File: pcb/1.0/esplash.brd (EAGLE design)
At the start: 101 x 71.1 mm, 64 parts, among them IC1 ACS712, K1 SRD-05VDC-SL-C, K2 SRD-05VDC-SL-C, K3 SRD-05VDC-SL-C, K4 SRD-05VDC-SL-C, Q1 BCX70SMD, Q2 BCX70SMD, Q3 BCX70SMD, Q4 BCX70SMD, U1 ESP-WROOM-32, U2 EL817(S)(D)(TU)-V, U3 EL817(S)(D)(TU)-V, U4 EL817(S)(D)(TU)-V, U5 EL817(S)(D)(TU)-V, Y1 ECS-.327-12.5-13X

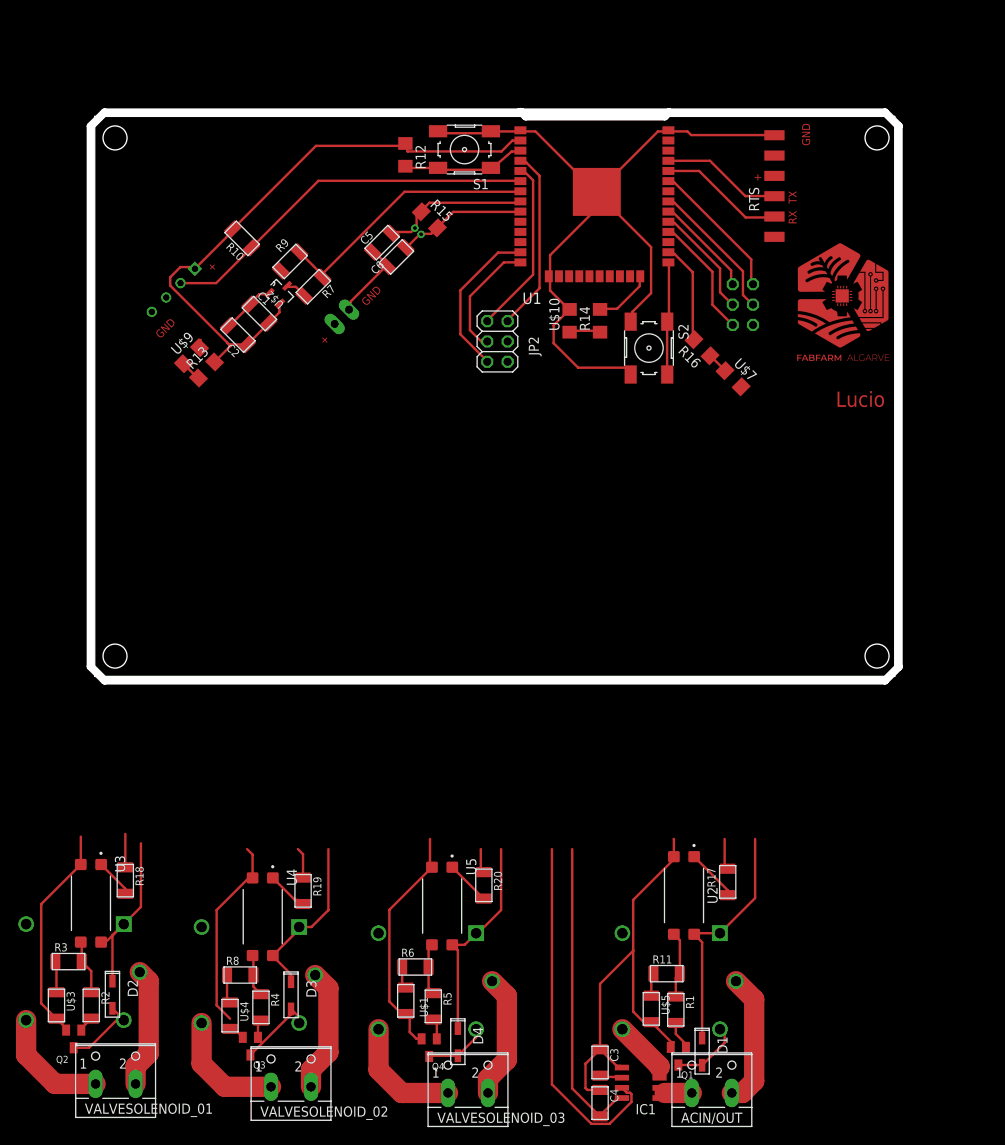
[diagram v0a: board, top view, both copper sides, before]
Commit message: PCB changes
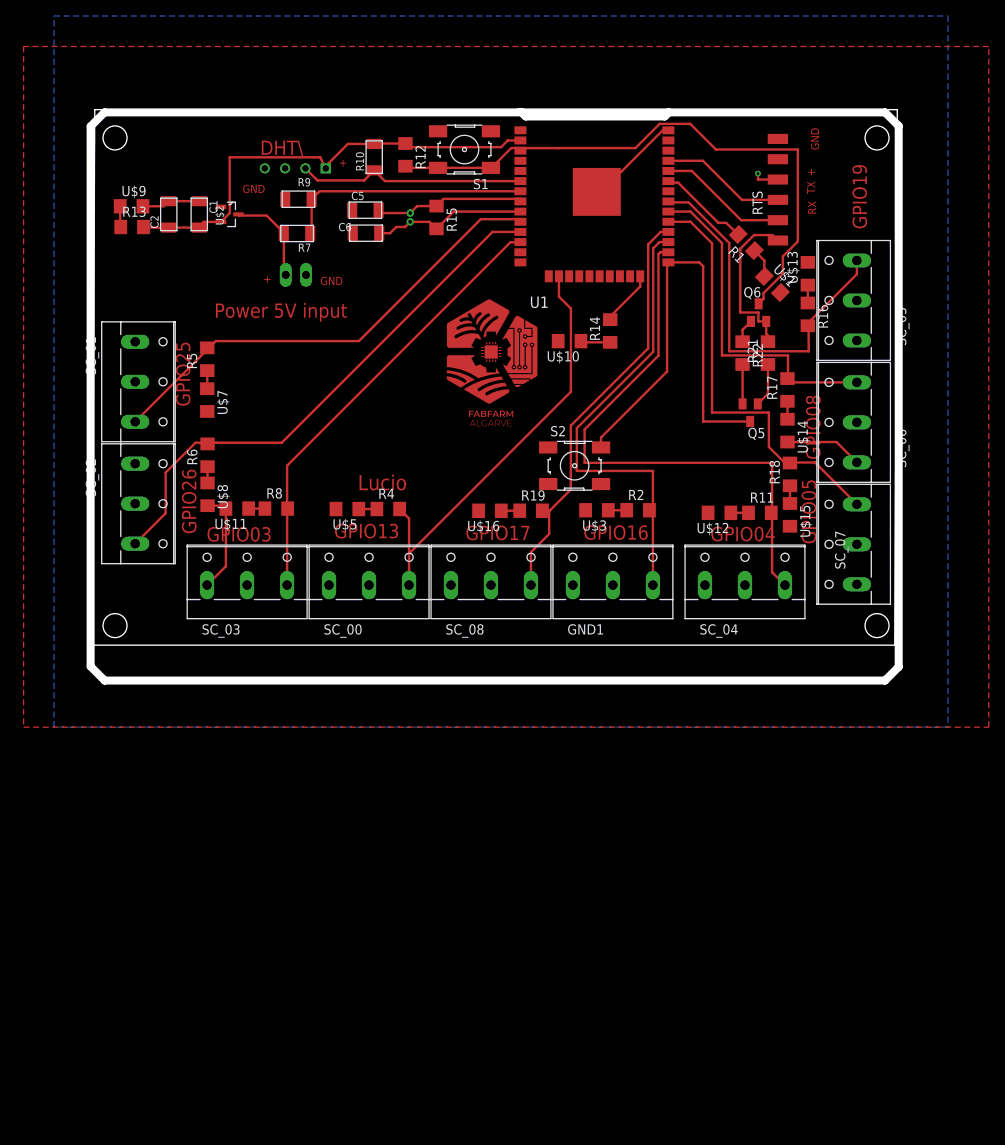
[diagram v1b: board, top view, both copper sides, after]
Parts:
- removed ACIN/OUT, VALVESOLENOID_01, VALVESOLENOID_02, VALVESOLENOID_03: (no value), con-wago-500:W237-102
- removed C3: 1nF, fab:C1206FAB
- removed C4: 0.1uF, fab:C1206FAB
- removed D1, D2, D3, D4: (no value), fab:SOD123
- removed IC1: ACS712, ACS712:SO08
- removed JP1, JP2: header2x6, pinhead:2X03
- removed K1, K2, K3, K4: SRD-05VDC-SL-C, SRD-05VDC-SL-C:RELAY_SRD-05VDC-SL-C
- removed Q1, Q2, Q3, Q4: BCX70SMD, transistor:SOT23
- removed R20: 220omh, fab:R1206FAB
- removed R3: 150ohm, fab:R1206FAB
- removed U$4: LEDFAB1206, fab:LED1206FAB
- removed U2, U3, U4, U5: EL817(S)(D)(TU)-V, EL817_S__D__TU_-V:SOIC254P1030X460-4N
- added GND1, SC_00, SC_01, SC_02, SC_03, SC_04, SC_05, SC_06, SC_07, SC_08: SC, con-wago-500:W237-103
- added Q5, Q6: BCX70SMD, transistor:SOT23
- added R21, R22: 10k, fab:R1206
- added U$11, U$12, U$13, U$14, U$15, U$16, U$8: LED, fab:LED1206
- R1, R2, R4, R5: value 1K -> 100ohm; device fab:R1206FAB -> fab:R1206
- R11: value 150ohm -> 100ohm; device fab:R1206FAB -> fab:R1206
- R17, R18, R19: value 220omh -> 100ohm; device fab:R1206FAB -> fab:R1206
- R6, R8: device fab:R1206FAB -> fab:R1206
- U$1, U$3, U$5: value LEDFAB1206 -> LED; device fab:LED1206FAB -> fab:LED1206
- moved U$1 100.6 mm to (84.7, 49.0), turned to 315 degrees
- moved R18 97.4 mm to (86.9, 25.2), turned to 90 degrees
- moved R1 96.3 mm to (81.4, 54.2), turned to 135 degrees
- moved R2 92.2 mm to (67.9, 20.8), turned to 0 degrees
- moved U$3 91.6 mm to (62.8, 20.8), turned to 180 degrees
- moved R5 85.7 mm to (14.1, 39.6), turned to 90 degrees
- moved U$5 73.1 mm to (31.6, 20.9), turned to 180 degrees
- moved R6 69.0 mm to (14.1, 27.6), turned to 90 degrees
- moved U$7 65.8 mm to (14.1, 34.5), turned to 270 degrees
- moved R4 64.3 mm to (36.7, 20.9), turned to 0 degrees
- moved R17 62.0 mm to (86.6, 35.8), turned to 90 degrees
- moved R11 58.8 mm to (83.1, 20.4)
- moved R8 58.5 mm to (22.7, 21.0)
- moved R19 55.4 mm to (54.5, 20.7), turned to 0 degrees
- moved U$6 21.6 mm to (25.1, 63.5), turned to 0 degrees
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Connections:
- removed net ACIN: ACIN/OUT.2, K2.COM
- removed net AMP_METER/IN: IC1.3, IC1.4, K2.NO
- removed net AMP_METER/OUT: ACIN/OUT.1, IC1.1, IC1.2
- removed net DELETE: C3.2, IC1.6
- removed net GPIO05: JP1.4, U1.29
- removed net GPIO17: JP1.6, U1.28
- removed net GPIO18: JP1.2, U1.30
- removed net GPIO19: JP1.3, U1.31
- removed net GPIO21: JP1.1, U1.33
- removed net N$12: K1.NO, VALVESOLENOID_01.1
- removed net N$14: R2.1, R3.2, U3.3
- removed net N$16: Q3.1, R4.2
- removed net N$18: R4.1, R8.2, U4.3
- removed net N$20: K4.COM, VALVESOLENOID_03.2
- removed net N$22: R6.1, U$1.1
- removed net N$24: K4.NO, VALVESOLENOID_03.1
- removed net N$28: JP2.3
- removed net N$30: R17.2, U2.1
- removed net N$32: R19.2, U4.1
- removed net N$33: R20.2, U5.1
- removed net N$43: Q1.1, R1.2
- removed net N$7: Q2.1, R2.2
- removed net N$8: R11.1, U$5.1
- removed net PUMPRELAYSEGMENT: D1.ANODE, K2.A2, Q1.3
- removed net RELAY1SEGMENT: D2.ANODE, K1.A2, Q2.3
- removed net RELAY2SEGMENT: D3.ANODE, K3.A2, Q3.3
- removed net RELAY3SEGMENT: D4.ANODE, K4.A2, Q4.3
- new net DTR: Q5.2, R22.2
- new net GPIO05/VALVE_RELAY07: R18.2, SC_07.3, U1.29
- new net GPIO17/VALVE_RELAY08: R19.2, SC_08.3, U1.28
- new net GPIO18/VALVE_RELAY06: R17.2, SC_06.3, U1.30
- new net GPIO19/VALVE_RELAY05: R16.2, SC_05.3, U1.31
- new net GPIO21/VALVE_RELAY04: R1.2, U1.33
- new net N$26: Q5.1, R21.1
- new net N$34: Q6.1, R22.1
- net CHIP_PU: now also Q6.3
- net GND: now also GND1.1, SC_00.1, SC_01.1, SC_02.1, SC_03.1, SC_04.1, SC_05.1, SC_06.1, SC_07.1, SC_08.1, U$11.2, U$12.2, U$13.2, U$14.2, U$15.2, U$16.2, U$8.2; no longer C3.1, C4.1, IC1.5, Q1.2, Q2.2, Q3.2, Q4.2, U$4.2, U2.2, U3.2, U4.2, U5.2
- net GPIO0: now also Q5.3
- net GPIO12: no longer JP2.4
- net GPIO13/PUMP_RELAY: now also R4.2, SC_00.3; no longer R17.1
- net GPIO14: no longer JP2.2
- net GPIO16/CURRENT_SENSE: now also GND1.3, R2.2; no longer IC1.7
- net GPIO25/VALVE_RELAY01: now also R5.2, SC_01.3; no longer R18.1
- net GPIO26/VALVE_RELAY02: now also R6.2, SC_02.3; no longer R19.1
- net GPIO27/VALVE_RELAY03: now also R8.2, SC_03.3; no longer R20.1
- net GPIO36: no longer JP2.5
- net GPIO39: no longer JP2.6
- net GPIO4: now also R11.2, SC_04.3; no longer R16.2
- net N$13: now also R4.1, U$5.1; no longer R3.1, U$3.1
- net N$15: now also R5.1, U$7.1; no longer K3.COM, VALVESOLENOID_02.2
- net N$17: now also R6.1, U$8.1; no longer R8.1, U$4.1
- net N$19: now also R8.1, U$11.1; no longer K3.NO, VALVESOLENOID_02.1
- net N$2: now also U$1.1; no longer R11.2, U2.3
- net N$21: now also R11.1, U$12.1; no longer Q4.1, R5.2
- net N$23: now also R16.1, U$13.1; no longer R5.1, R6.2, U5.3
- net N$27: now also R17.1, U$14.1; no longer JP2.1
- net N$29: now also R18.1, U$15.1; no longer R16.1, U$7.1
- net N$31: now also R19.1, U$16.1; no longer R18.2, U3.1
- net N$5: now also R2.1, U$3.1; no longer K1.COM, VALVESOLENOID_01.2
- net RTS: now also Q6.2, R21.2
- net VCC: now also GND1.2, SC_00.2, SC_01.2, SC_02.2, SC_03.2, SC_04.2, SC_05.2, SC_06.2, SC_07.2, SC_08.2; no longer C4.2, D1.CATHODE, D2.CATHODE, D3.CATHODE, D4.CATHODE, IC1.8, K1.A1, K2.A1, K3.A1, K4.A1, U2.4, U3.4, U4.4, U5.4
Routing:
- net GND: track 265.7 -> 42.9 mm
- net VCC: track 141.5 -> 15.2 mm, vias 0 -> 1
- net GPIO26/VALVE_RELAY02: track 3.83 -> 67.5 mm
- net GPIO4: track 12.6 -> 70.8 mm
- net CHIP_PU: track 16.8 -> 74.3 mm
- net GPIO25/VALVE_RELAY01: track 4.18 -> 59.0 mm
- net GPIO05/VALVE_RELAY07: track 0.00 -> 53.5 mm
- net GPIO27/VALVE_RELAY03: track 3.03 -> 55.8 mm
- net GPIO17/VALVE_RELAY08: track 0.00 -> 52.7 mm
- net GPIO13/PUMP_RELAY: track 3.88 -> 53.7 mm
- net GPIO19/VALVE_RELAY05: track 0.00 -> 47.3 mm
- net GPIO18/VALVE_RELAY06: track 0.00 -> 42.7 mm
- net GPIO0: track 14.2 -> 56.5 mm
- net GPIO36: track 23.1 -> 0.00 mm
- net GPIO39: track 22.1 -> 0.00 mm
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- added copper zone on layer 1, net GND
- added copper zone on layer 16, net VCC
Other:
- board size 101 x 71.1 mm -> 101 x 71.4 mm
- board text added: "DHT\"
- board text added: "GPIO03"
- board text added: "GPIO04"
- board text added: "GPIO05"
- board text added: "GPIO08"
- board text added: "GPIO13"
- board text added: "GPIO16"
- board text added: "GPIO17"
- board text added: "GPIO19"
- board text added: "GPIO25"
- board text added: "GPIO26"
- board text added: "Power 5V input"
